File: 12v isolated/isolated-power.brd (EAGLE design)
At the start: 53.3 x 41.6 mm, 10 parts, among them Q1 SPW47N60S5, Q2 SPW47N60S5

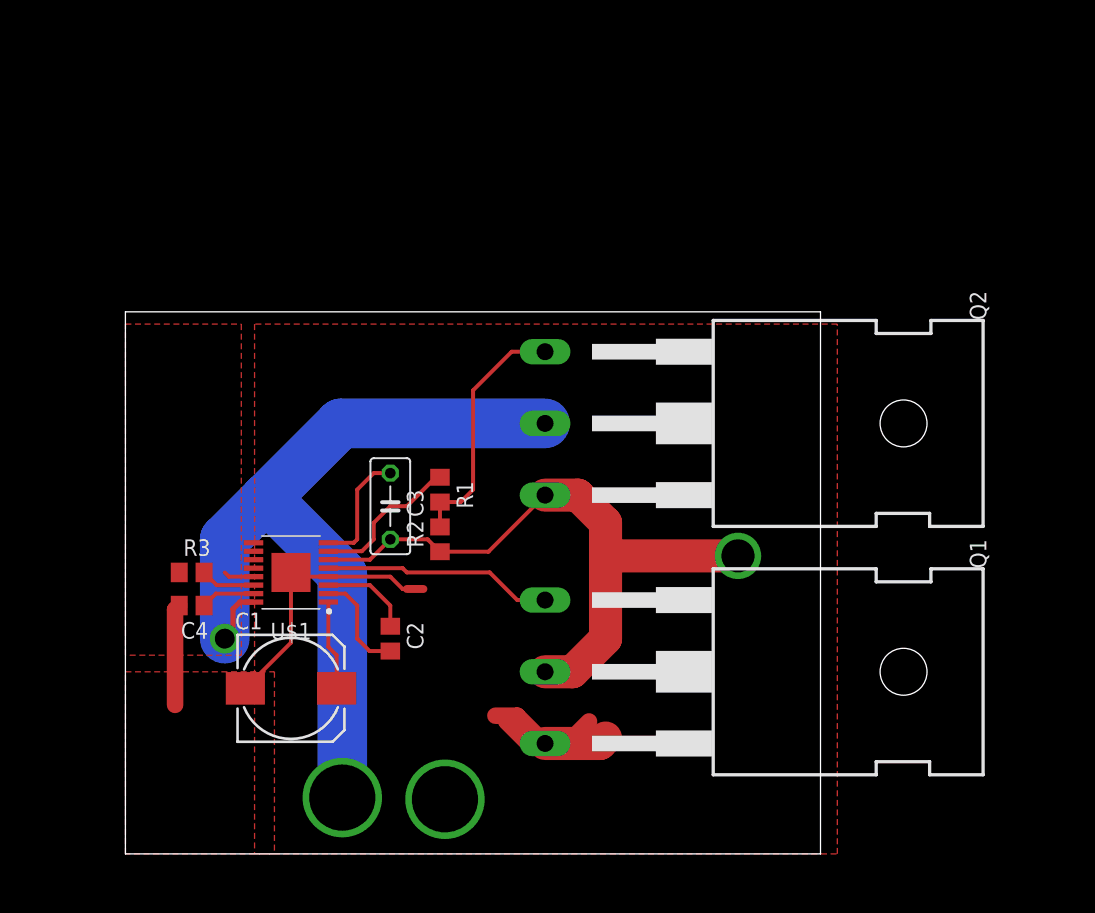
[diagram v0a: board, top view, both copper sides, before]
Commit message: production files
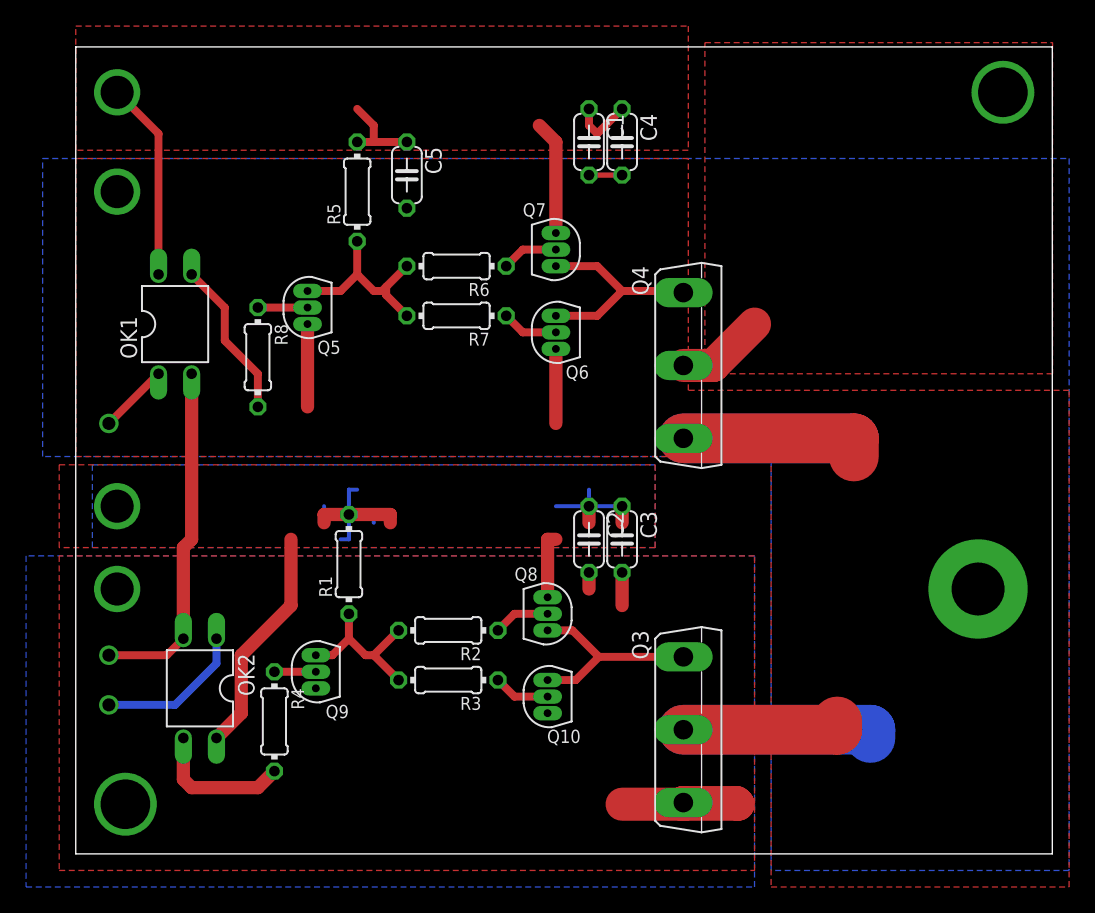
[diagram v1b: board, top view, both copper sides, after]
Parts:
- removed Q1, Q2: SPW47N60S5, transistor-fet:P-TO247
- removed U$1: A3946KLPTR-T, MotorDriver:SOP65P640X120-17T300
- added C5: (no value), rcl:C050-024X044
- added OK1, OK2: LTV816, optocoupler:DIL04
- added Q10, Q5, Q6, Q9: 2N3904, transistors:TO-92
- added Q3, Q4: IRFPC40, transistor-power:TO247BV
- added Q7, Q8: 2N3906, transistors:TO-92
- added R4: (no value), rcl:0204/7
- added R5, R6, R7: 500r, rcl:0204/7
- added R8: 1k, rcl:0204/7
- C1: value 10uF 25V -> 0.1u; device rcl:175TMP-0808 -> rcl:C050-024X044
- C2: value 0.47uF -> 0.1u; device rcl:C0805 -> rcl:C050-024X044
- C3: value 0.47uF -> 1u; device rcl:C050-030X075 -> rcl:C050-024X044
- C4: value 0.1uF -> 1u; device rcl:C0805 -> rcl:C050-024X044
- R1: value (none) -> 1k; device rcl:R0805 -> rcl:0204/7
- R2: device rcl:R0805 -> rcl:0204/7
- R3: value 80k -> (none); device rcl:R0805 -> rcl:0204/7
- moved C4 48.5 mm to (38.1, 54.6), turned to 270 degrees
- moved C1 47.7 mm to (35.6, 54.6), turned to 270 degrees
- moved R3 21.3 mm to (24.8, 13.3), turned to 180 degrees
- moved C3 18.0 mm to (38.1, 24.1)
- moved C2 17.0 mm to (35.6, 24.1)
- moved R1 9.03 mm to (17.1, 22.2), turned to 90 degrees
- moved R2 7.01 mm to (24.8, 17.1), turned to 180 degrees
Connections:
- removed net AGND: C1.-, C4.2, Q1.3, R3.1, U$1.LGND, U$1.PAD, U$1.PGND
- new net 12V-HIGH: C1.1, C4.1, C5.1, OK1.4, Q7.E, R5.2
- new net 12V-LOW: C2.1, C3.1, OK2.4, Q8.E, R1.2
- new net GND: C2.2, C3.2, Q10.E, Q3.S, Q9.E
- new net GND1: OK1.2, OK2.2
- new net MOTOR_OUT: C1.2, C4.2, C5.2, Q3.D, Q4.S, Q5.E, Q6.E
- net N$1: now also Q10.C, Q3.G, Q8.C; no longer C2.2, U$1.CP2
- net N$10: now also Q7.B, R6.1; no longer R3.2, U$1.DT
- net N$11: now also Q6.B, R7.1; no longer U$1.RESET
- net N$12: now also Q5.B, R8.1; no longer U$1.IN2
- net N$13: now also OK2.1; no longer U$1.IN1
- net N$14: now also OK1.1; no longer U$1.FAULT
- net N$2: now also Q9.C, R1.1, R2.2, R3.2; no longer C1.+, U$1.VREG
- net N$3: now also OK1.3, R8.2; no longer C2.1, U$1.CP1
- net N$4: now also Q8.B, R2.1; no longer Q1.1, U$1.GL
- net N$5: now also Q10.B, R3.1; no longer C3.2, Q1.2, Q2.3, R2.1, U$1.S
- net N$6: now also Q9.B, R4.1; no longer C3.1, U$1.BOOT
- net N$7: now also Q4.G, Q6.C, Q7.C; no longer R1.1, U$1.GH
- net N$8: now also Q5.C, R5.1, R6.2, R7.2; no longer Q2.1, R1.2, R2.2
- net N$9: now also OK2.3, R4.2; no longer C4.1, U$1.VREF
- net V+: now also Q4.D; no longer Q2.2, U$1.VBB
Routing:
- net MOTOR_OUT: track 0.00 -> 83.7 mm, vias 0 -> 2
- net V+: track 65.6 -> 6.78 mm, vias 2 -> 1
- net N$5: track 57.3 -> 4.34 mm, vias 1 -> 0
- net 12V-LOW: track 0.00 -> 50.6 mm, vias 0 -> 1
- net AGND: track 48.4 -> 0.00 mm, vias 1 -> 0
- net 12V-HIGH: track 0.00 -> 40.2 mm, vias 0 -> 1
- net GND1: track 0.00 -> 26.8 mm, vias 0 -> 1
- net GND: track 0.00 -> 17.0 mm, vias 0 -> 2
- net N$4: track 17.6 -> 4.34 mm
- net N$13: track 0.00 -> 11.5 mm, vias 0 -> 1
- net N$1: track 8.06 -> 15.9 mm
- net N$9: track 4.18 -> 10.9 mm
- net N$6: track 9.20 -> 3.18 mm
- net N$2: track 6.88 -> 12.8 mm
- net N$14: track 0.00 -> 5.39 mm, vias 0 -> 1
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- added copper zone on layer 1, net 12V-HIGH
- added copper zone on layer 1, net 12V-LOW
- added copper zone on layer 16, net 12V-LOW
- added copper zone on layer 1, net GND
- added copper zone on layer 16, net GND
- added copper zone on layer 1, net MOTOR_OUT
- added copper zone on layer 16, net MOTOR_OUT
- added copper zone on layer 1, net V+
- removed copper zone on layer 1, net AGND
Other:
- board size 53.3 x 41.6 mm -> 74.9 x 61.9 mm
